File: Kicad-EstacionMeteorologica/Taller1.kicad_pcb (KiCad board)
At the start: 2 copper layers, 85.7 x 137.2 mm, 10 parts, among them U1 DHT11, U4 SX1262-XIAO

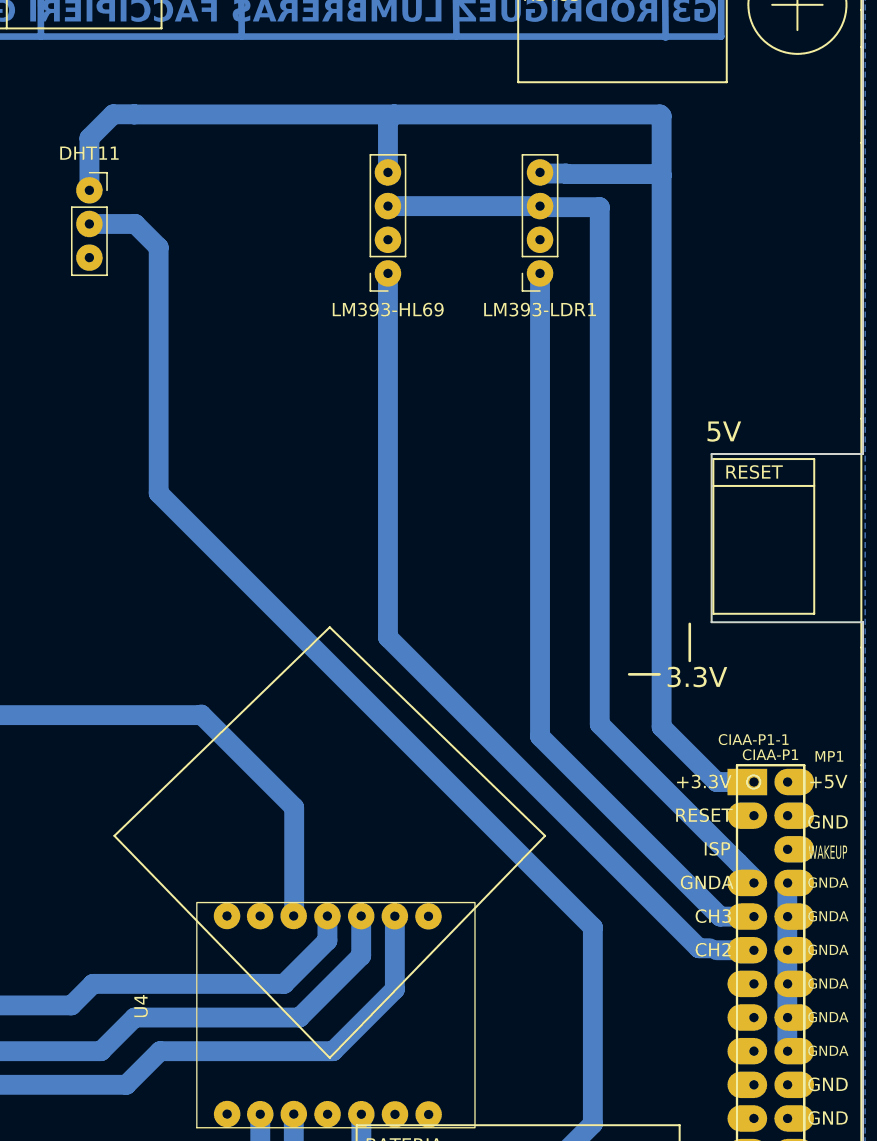
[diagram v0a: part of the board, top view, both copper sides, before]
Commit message: Ultima version pistas pulidas
Cambios de lolo.
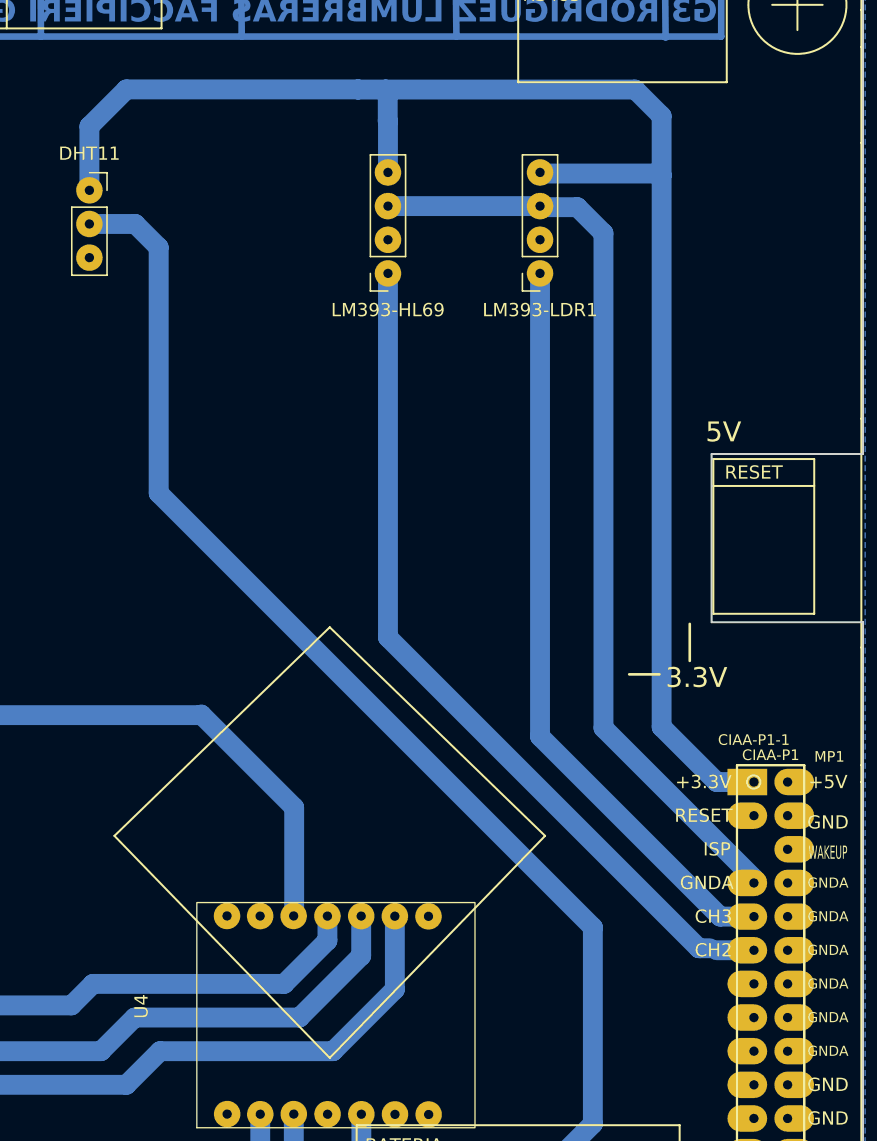
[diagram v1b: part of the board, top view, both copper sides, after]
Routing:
- net (no net): track 12.7 -> 0.00 mm
- net Alimentacion 3.3v: track 168.5 -> 172.3 mm
- net GNDA: track 71.2 -> 70.2 mm
